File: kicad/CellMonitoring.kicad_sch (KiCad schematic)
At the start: 57 parts, among them J7 Conn_01x04, U1 HDC3022, U11 TMCS1123x3, U12 DAC7571, U13 DAC7571, U14 TMCS1123x3, U17 LTC6803-4, U20 LTC6803-4, U21 LTC6803-4, U3 HDC3022, U4 HDC3022, U5 HDC3022, U6 HDC3022, U61 MLX90632

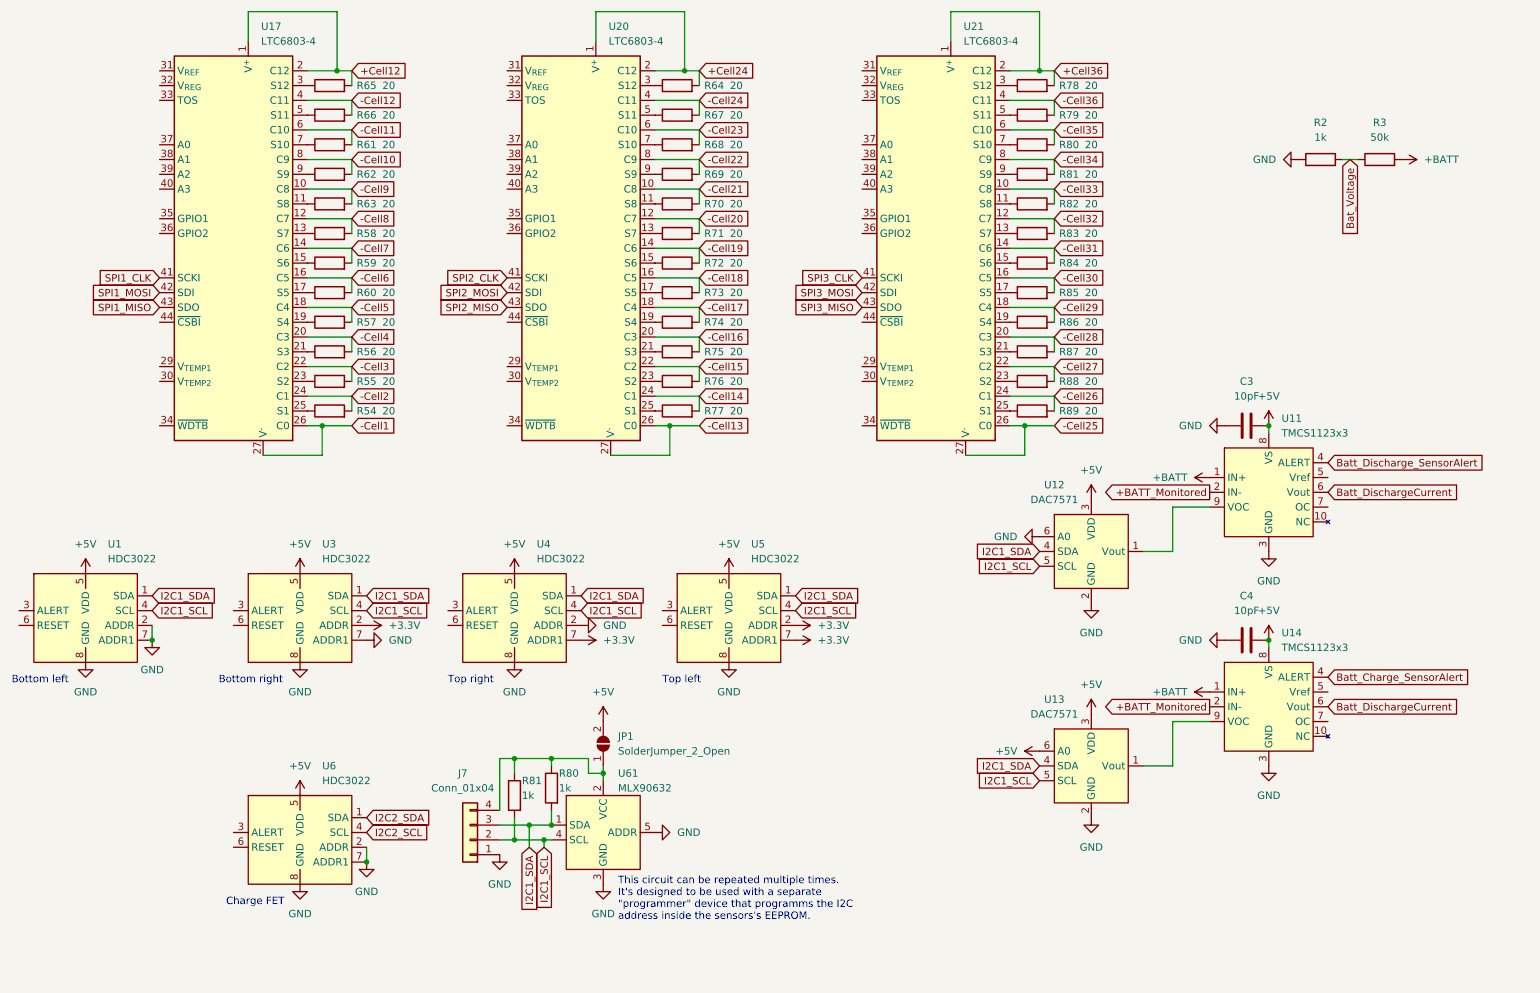
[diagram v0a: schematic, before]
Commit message: More refactors for the god of refactors
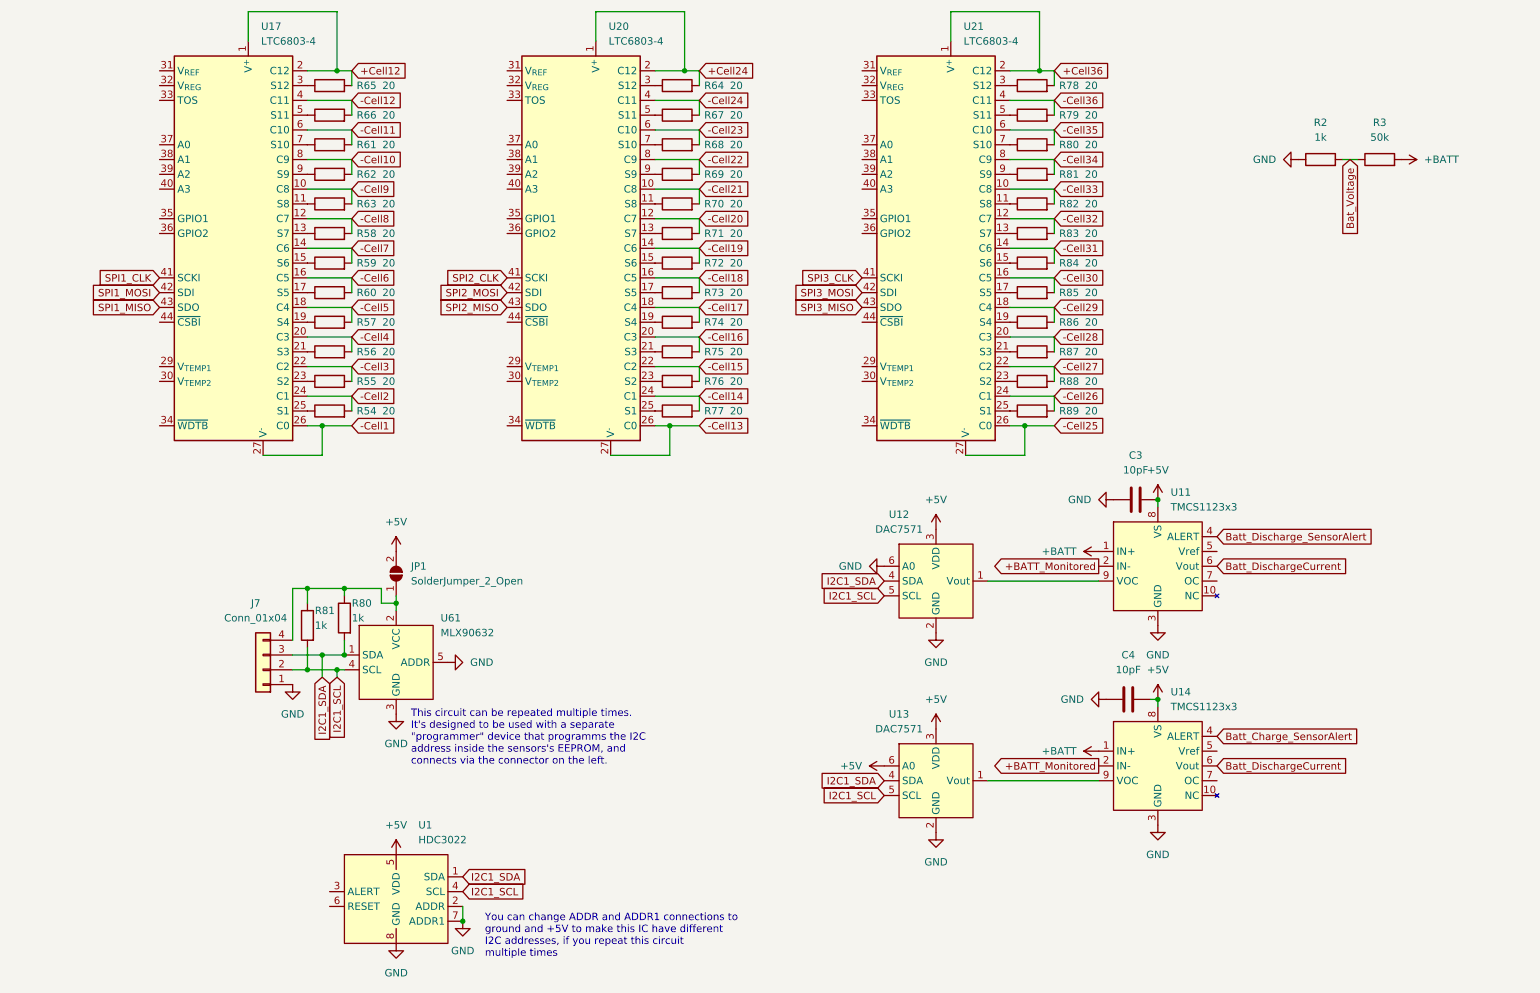
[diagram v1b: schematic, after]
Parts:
- removed U3, U4, U5, U6: HDC3022, Package_SON:Texas_S-PWSON-N8_EP1.2x2mm, symbol Sensor_Humidity:HDC3022
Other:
- note added: "This circuit can be repeated multiple times. It's designed to be used with a separate "programmer" device that programms the I2C address inside the sensors's EEPROM, and connects via the connector on the left."
- note added: "You can change ADDR and ADDR1 connections to ground and +5V to make this IC have different I2C addresses, if you repeat this circuit multiple times"
- note removed: "Bottom left"
- note removed: "Bottom right"
- note removed: "Charge FET"
- note removed: "This circuit can be repeated multiple times. It's designed to be used with a separate "programmer" device that programms the I2C address inside the sensors's EEPROM."
- note removed: "Top left"
- note removed: "Top right"
- moved on the sheet: C3, C4, J7, JP1, R80, R81, U1, U11, U12, U13, U14, U61
